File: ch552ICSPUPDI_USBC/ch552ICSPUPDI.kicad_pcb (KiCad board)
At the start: 2 copper layers, 22 x 34 mm, 21 parts, among them J1 USB_B_Micro, J2 PWR, J3 icsp, J4 UPDI, SW1 SW_SPST, U1 CH552G, U2 AMS1117-3.3

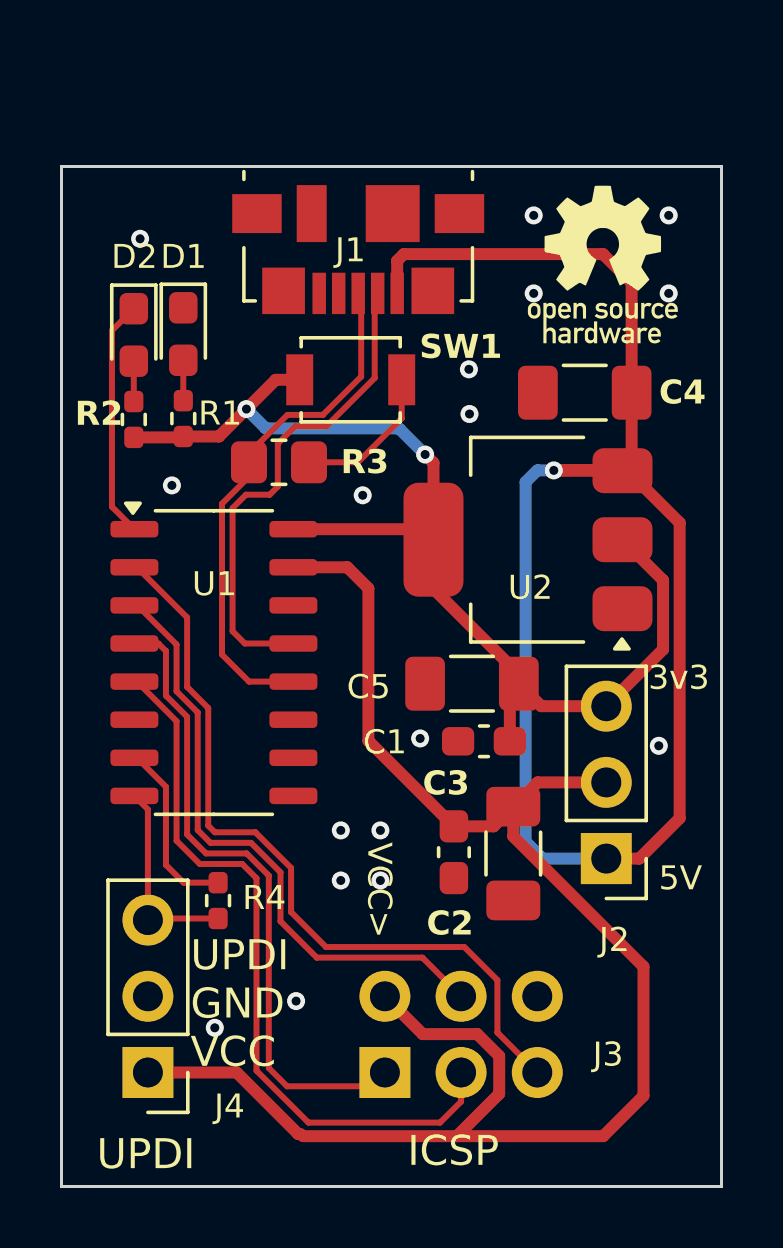
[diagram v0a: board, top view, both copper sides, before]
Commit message: update
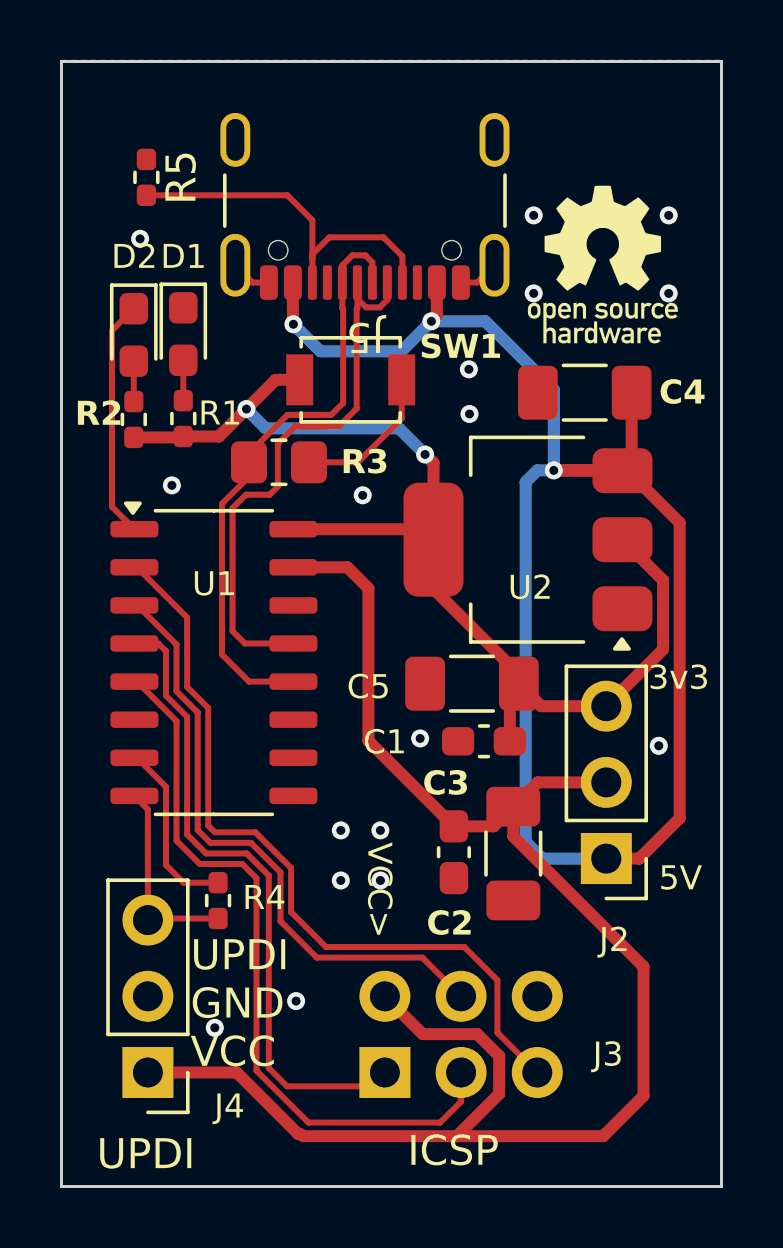
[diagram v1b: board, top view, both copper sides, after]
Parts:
- removed J1: USB_B_Micro, Connector_USB:USB_Micro-B_Molex_47346-0001
- added J5: USB_C_Receptacle_USB2.0_16P, Connector_USB:USB_C_Receptacle_GCT_USB4105-xx-A_16P_TopMnt_Horizontal, F.Cu at (126.9, 72.0)
- added R5: 5.1k, Resistor_SMD:R_0402_1005Metric_Pad0.72x0.64mm_HandSolder, F.Cu at (119.6, 72.2)
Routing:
- net Net-(J5-CC1): track 0.00 -> 12.5 mm
- net /D+: track 17.4 -> 21.1 mm
- net /D-: track 16.5 -> 20.1 mm
- net +5V: track 51.9 -> 54.7 mm, vias 1 -> 3
- net GND: track 0.51 -> 2.87 mm
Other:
- board size 22 x 34 mm -> 22 x 37.5 mm
